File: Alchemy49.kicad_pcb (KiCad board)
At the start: 2 copper layers, 267.5 x 76.2 mm, 255 parts, among them J1 USB_B_Micro, J2 Conn_01x05_Female, Q1 2N7002E, SW1 ESC-1.5U, SW10 O-1U, SW11 P-1U, SW12 BACK-1.5U, SW13 DEL-1U, SW14 TAB-1.75U, SW15 A-1U, SW16 S-1U, SW17 D-1U, SW18 F-1U, SW19 G-1U, SW2 Q-1U, SW20 H-1U, SW21 J-1U, SW22 K-1U, SW23 L-1U, SW24 ENTER-2.25U, SW25 PGUP-1U, SW26 SHIFT-2U, SW27 Z-1U, SW28 X-1U, SW29 C-1U, SW3 W-1U, SW30 V-1U, SW31 B-1U, SW32 N-1U, SW33 M-1U, SW34 COM-1U, SW35 PER-1U, SW36 SLASH-1U, SW37 UP-1U, SW38 PGDN-1U, SW39 CTRL1-1U, SW4 E-1U, SW40 WIN-1U, SW41 ALT-1U, SW42 FN1-1U, SW43 SPACE-2.75U, SW44 SHIFT-2.25U, SW45 FN2-1U, SW46 CTRL2-1U, SW47 LEFT-1U, SW48 DOWN-1U, SW49 RIGHT-1U, SW5 R-1U, SW6 T-1U, SW7 Y-1U, SW8 U-1U, SW9 I-1U

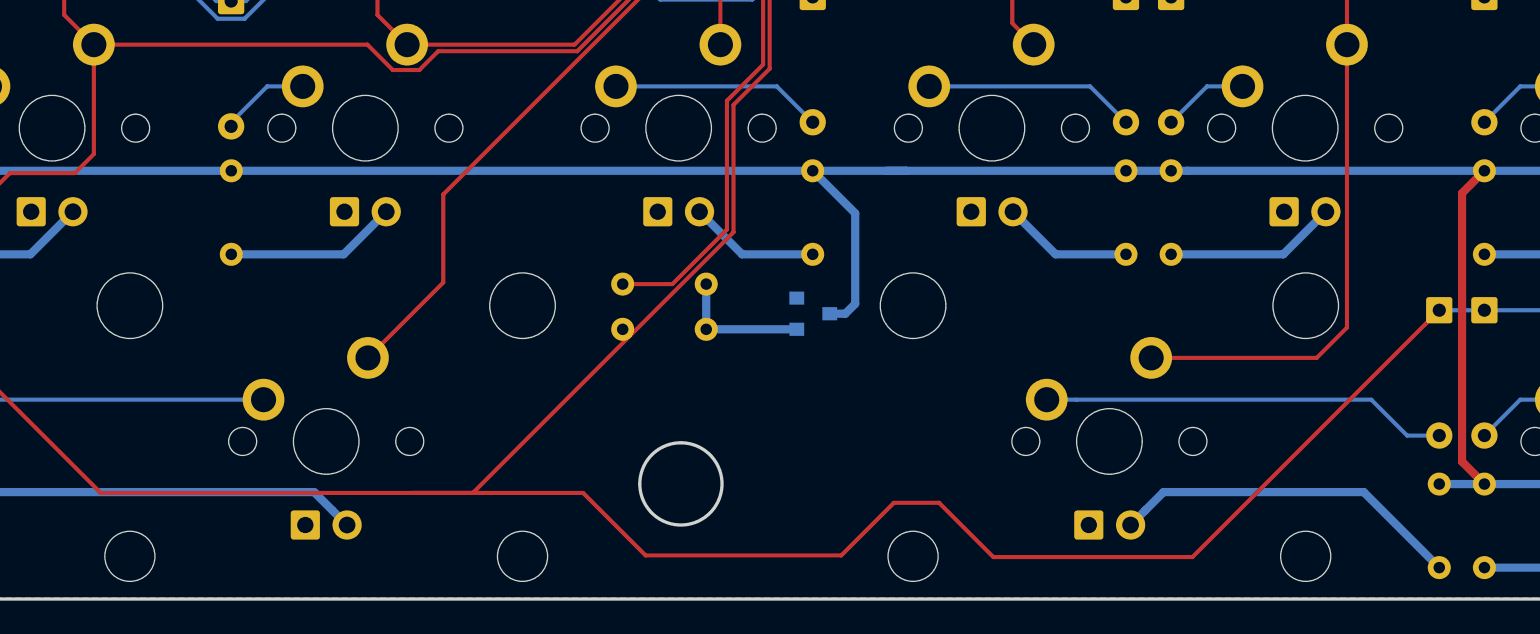
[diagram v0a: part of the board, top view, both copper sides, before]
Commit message: Finalized Board Design
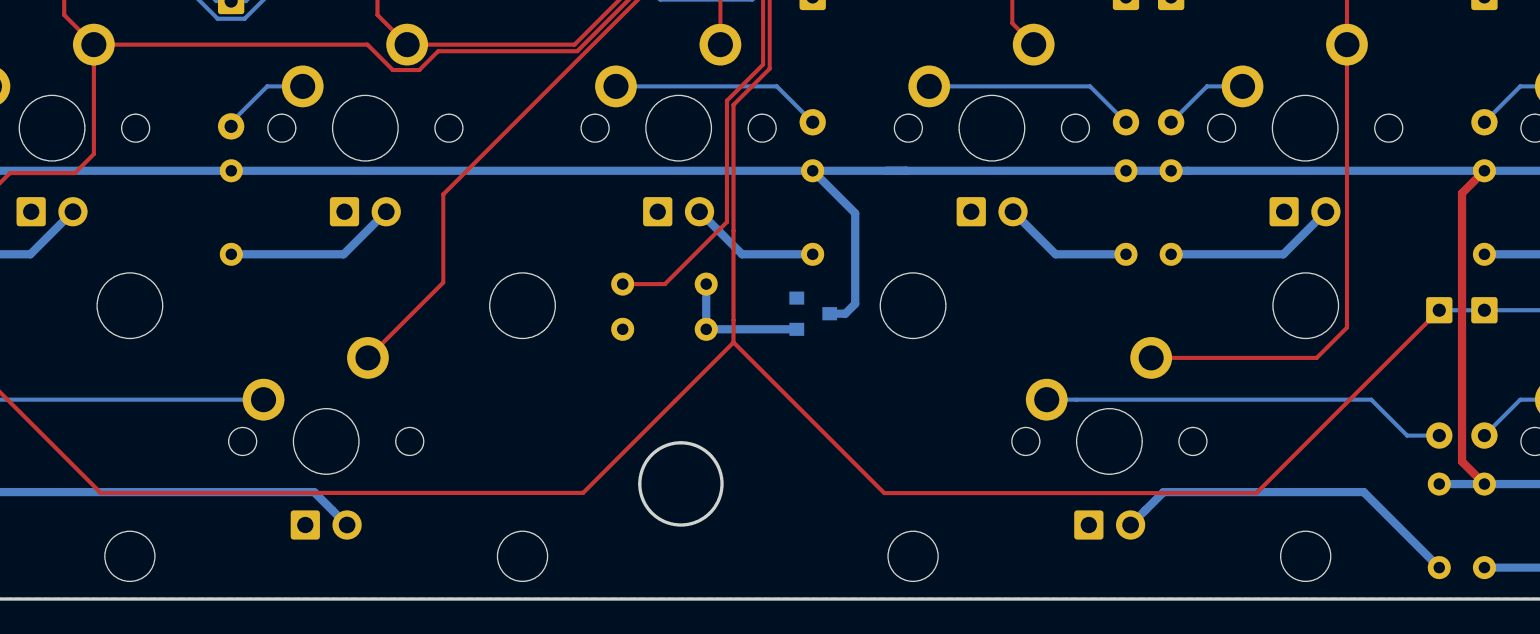
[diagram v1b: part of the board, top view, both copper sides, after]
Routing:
- net Row4: track 273.5 -> 255.8 mm
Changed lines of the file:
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@@
     (thickness 1.6)
     (drawings 24)
-    (tracks 831)
+    (tracks 827)
     (zones 0)
     (modules 255)
@@
   (segment (start 206.16 72.19) (end 225.21 72.19) (width 0.25) (layer B.Cu) (net 8))
   (segment (start 225.21 72.19) (end 241.515 72.19) (width 0.25) (layer B.Cu) (net 8))
-  (segment (start 136.1 87.1) (end 132.3 83.3) (width 0.25) (layer F.Cu) (net 8))
-  (segment (start 184.365 72.19) (end 169.355 87.2) (width 0.25) (layer F.Cu) (net 8))
-  (segment (start 169.355 87.2) (end 157.25 87.2) (width 0.25) (layer F.Cu) (net 8))
-  (segment (start 157.25 87.2) (end 153.95 83.9) (width 0.25) (layer F.Cu) (net 8))
-  (segment (start 153.95 83.9) (end 151.2 83.9) (width 0.25) (layer F.Cu) (net 8))
-  (segment (start 151.2 83.9) (end 148 87.1) (width 0.25) (layer F.Cu) (net 8))
-  (segment (start 148 87.1) (end 136.1 87.1) (width 0.25) (layer F.Cu) (net 8))
-  (segment (start 130.35 83.3) (end 132.3 83.3) (width 0.25) (layer F.Cu) (net 8))
   (segment (start 34.49 71.59) (end 35.09 72.19) (width 0.25) (layer B.Cu) (net 8))
   (segment (start 31.965 71.59) (end 34.49 71.59) (width 0.25) (layer B.Cu) (net 8))
   (segment (start 35.09 72.19) (end 50.115 72.19) (width 0.25) (layer B.Cu) (net 8))
   (segment (start 91.86 72.19) (end 102.97 83.3) (width 0.25) (layer F.Cu) (net 8))
-  (segment (start 102.97 83.3) (end 107.825 83.3) (width 0.25) (layer F.Cu) (net 8))
-  (segment (start 125.596999 83.3) (end 121.9 83.3) (width 0.25) (layer F.Cu) (net 8))
-  (segment (start 121.9 83.3) (end 130.35 83.3) (width 0.25) (layer F.Cu) (net 8))
-  (segment (start 107.825 83.3) (end 121.9 83.3) (width 0.25) (layer F.Cu) (net 8))
+  (segment (start 137.89699 77.70301) (end 132.3 83.3) (width 0.25) (layer F.Cu) (net 8))
+  (segment (start 141.45 74.15) (end 137.89699 77.70301) (width 0.25) (layer F.Cu) (net 8))
+  (segment (start 143.65 57.5) (end 141.45 59.7) (width 0.25) (layer F.Cu) (net 8))
   (segment (start 145.14 49.37) (end 143.65 50.86) (width 0.25) (layer F.Cu) (net 8))
   (segment (start 143.65 50.86) (end 143.65 57.5) (width 0.25) (layer F.Cu) (net 8))
-  (segment (start 141.45 67.446999) (end 125.596999 83.3) (width 0.25) (layer F.Cu) (net 8))
-  (segment (start 143.65 57.5) (end 141.45 59.7) (width 0.25) (layer F.Cu) (net 8))
-  (segment (start 141.45 59.7) (end 141.45 67.446999) (width 0.25) (layer F.Cu) (net 8))
+  (segment (start 102.97 83.3) (end 132.3 83.3) (width 0.25) (layer F.Cu) (net 8))
+  (segment (start 141.45 72.79) (end 141.45 74.15) (width 0.25) (layer F.Cu) (net 8))
+  (segment (start 141.45 67.35) (end 141.45 72.79) (width 0.25) (layer F.Cu) (net 8))
+  (segment (start 141.45 59.7) (end 141.45 67.35) (width 0.25) (layer F.Cu) (net 8))
+  (segment (start 141.46 74.15) (end 141.45 74.15) (width 0.25) (layer F.Cu) (net 8))
+  (segment (start 150.62 83.31) (end 141.46 74.15) (width 0.25) (layer F.Cu) (net 8))
+  (segment (start 184.365 72.19) (end 173.245 83.31) (width 0.25) (layer F.Cu) (net 8))
+  (segment (start 173.245 83.31) (end 150.62 83.31) (width 0.25) (layer F.Cu) (net 8))
   (segment (start 103.56625 20.47875) (end 105.7275 20.47875) (width 0.25) (layer B.Cu) (net 9))
   (segment (start 101.385 22.66) (end 103.56625 20.47875) (width 0.25) (layer B.Cu) (net 9))
@@
   (segment (start 148.25 72.4) (end 148.85 71.8) (width 0.5) (layer B.Cu) (net 124))
   (segment (start 147.3 72.4) (end 148.25 72.4) (width 0.5) (layer B.Cu) (net 124))
-  (segment (start 137.7313 70.6) (end 134.66 70.6) (width 0.25) (layer F.Cu) (net 125))
-  (segment (start 141.04999 67.28131) (end 137.7313 70.6) (width 0.25) (layer F.Cu) (net 125))
-  (segment (start 141.04999 59.45001) (end 141.04999 67.28131) (width 0.25) (layer F.Cu) (net 125))
   (segment (start 143.24999 57.25001) (end 141.04999 59.45001) (width 0.25) (layer F.Cu) (net 125))
   (segment (start 148.975199 48.225199) (end 144.526895 48.225199) (width 0.25) (layer F.Cu) (net 125))
@@
   (segment (start 143.895199 50.049102) (end 143.24999 50.694311) (width 0.25) (layer F.Cu) (net 125))
   (segment (start 143.24999 50.694311) (end 143.24999 57.25001) (width 0.25) (layer F.Cu) (net 125))
+  (segment (start 141.04999 59.45001) (end 141.04999 66.83001) (width 0.25) (layer F.Cu) (net 125))
+  (segment (start 137.28 70.6) (end 141.04999 66.83001) (width 0.25) (layer F.Cu) (net 125))
+  (segment (start 134.71 70.6) (end 137.28 70.6) (width 0.25) (layer F.Cu) (net 125))
   (segment (start 145.3 73.35) (end 139.79 73.35) (width 0.5) (layer B.Cu) (net 126))
   (segment (start 139.79 70.6) (end 139.79 73.35) (width 0.5) (layer B.Cu) (net 126))
